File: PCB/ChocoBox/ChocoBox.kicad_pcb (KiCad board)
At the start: 2 copper layers, 101.6 x 61.5 mm, 27 parts, among them J1 DTH22_01, J10 Vout-12V, J11 Conn_01x01, J12 I2C, J13 I2C, J14 Vout-5V-Humidificador, J15 Conn_01x01, J16 Conn_01x01, J17 Conn_01x01, J18 Conn_01x01, J19 DS18B20-A, J2 DTH22_02, J20 DS18B20-B, J21 DS18B20-C, J22 DS18B20-D, J3 DS3231, J4 LCD2004A, J5 microSD, J6 Humidificador, J7 WaterLevel, J8 Vin-12V, J9 Calentador, SW1 BTN1, U1 ESP32-DEVKIT-V1, U2 DCDC_StepDown_LM2596

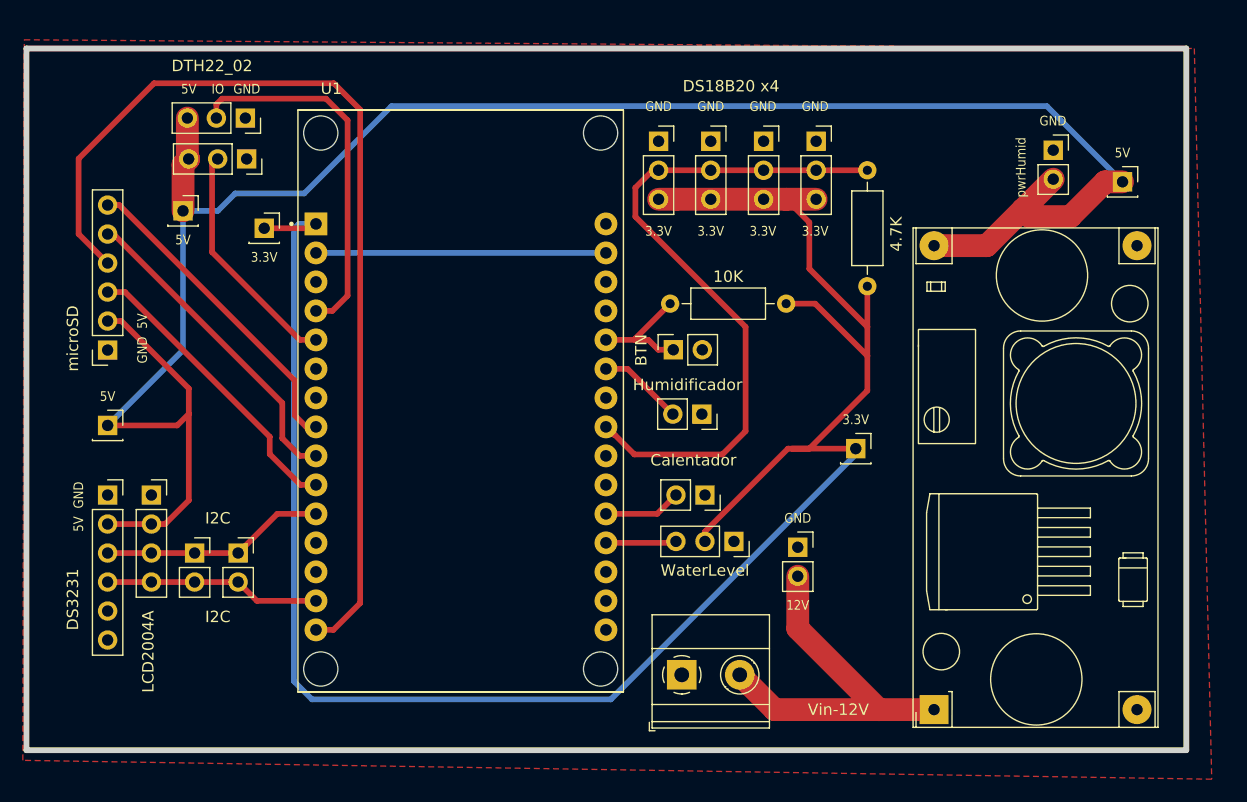
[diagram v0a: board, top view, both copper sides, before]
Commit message: controladores funcionando
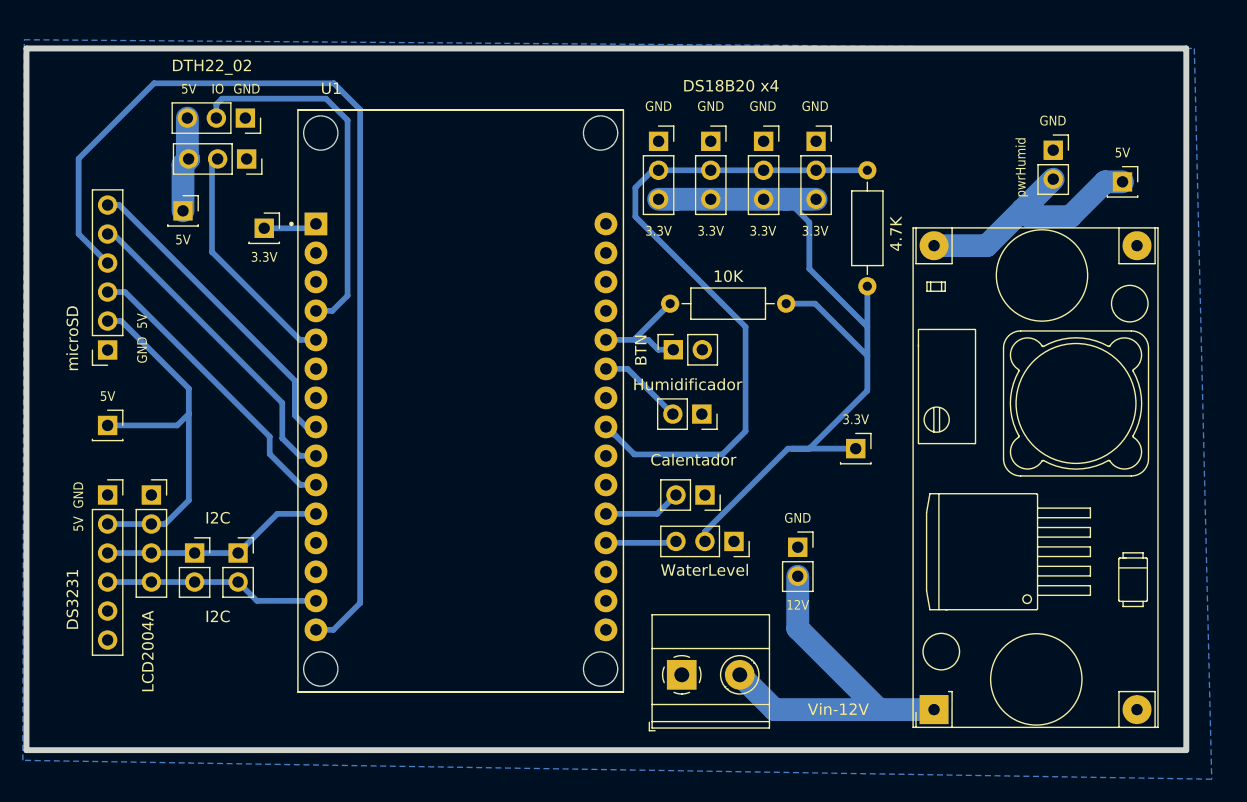
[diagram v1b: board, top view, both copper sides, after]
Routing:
- net +5V: track 176.7 -> 66.3 mm
- net +3.3V: track 176.5 -> 76.0 mm
- net GND: track 25.4 -> 0.00 mm
- added copper zone on B.Cu, net GND
- removed copper zone on F.Cu, net GND

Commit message: Bug fix - App environment.txt
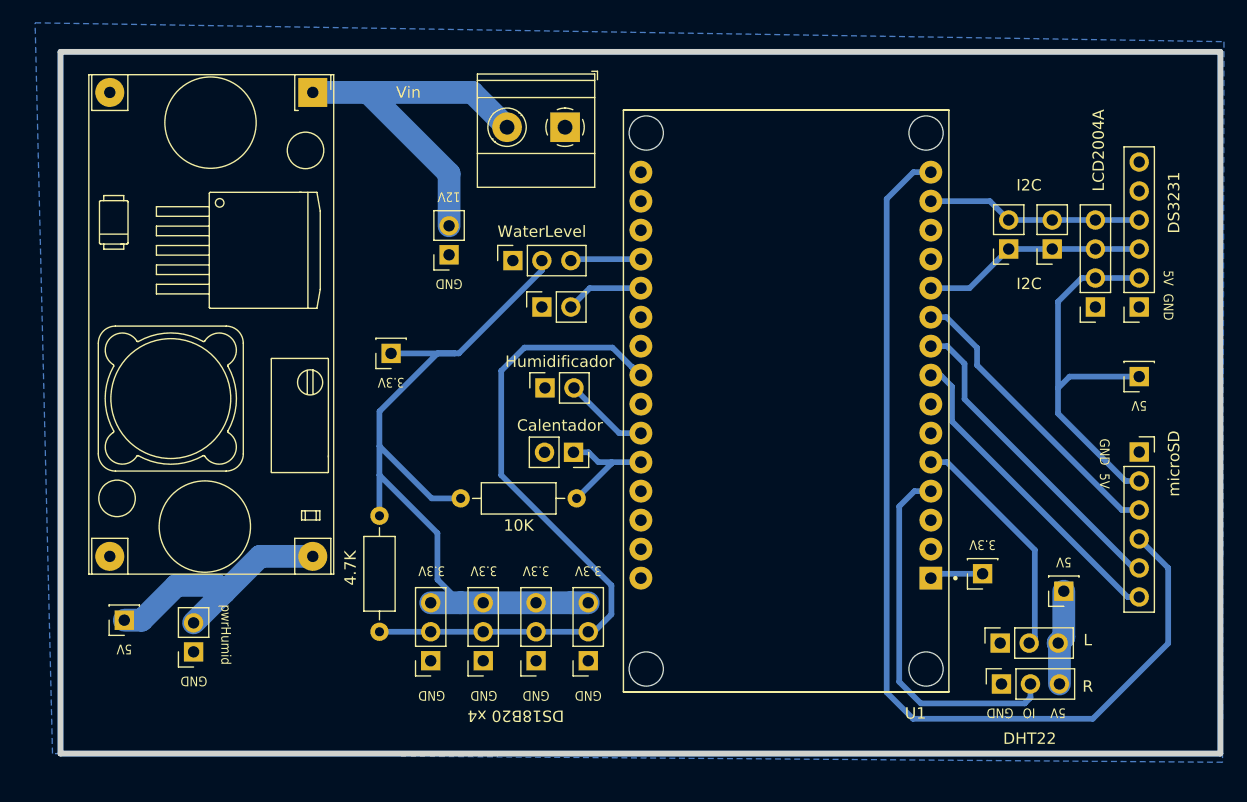
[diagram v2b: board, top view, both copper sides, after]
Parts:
- J2: value DTH22_02 -> R
- J8: value Vin-12V -> Vin
- moved J16 95.5 mm to (70.0, 87.2), turned to 180 degrees
- moved J3 91.8 mm to (158.9, 59.7), turned to 180 degrees
- moved J5 90.8 mm to (158.9, 72.4), turned to 0 degrees
- moved J15 90.5 mm to (158.9, 65.8), turned to 180 degrees
- moved J14 87.2 mm to (76.1, 89.9), turned to 180 degrees
- moved J4 84.3 mm to (155.1, 59.7), turned to 180 degrees
- moved J11 84.0 mm to (152.3, 84.6), turned to 180 degrees
- moved J2 82.7 mm to (146.9, 92.8), turned to 90 degrees
- moved J12 79.7 mm to (151.3, 54.6), turned to 180 degrees
- moved J1 78.5 mm to (146.8, 89.2), turned to 90 degrees
- moved U2 76.7 mm to (86.5, 40.9), turned to -90 degrees
- moved J13 72.6 mm to (147.5, 54.6), turned to 180 degrees
- moved J18 69.8 mm to (145.2, 83.1), turned to 180 degrees
- moved R3 58.8 mm to (92.4, 88.2), turned to 90 degrees
- moved J22 56.7 mm to (96.9, 90.7), turned to 180 degrees
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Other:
- board text added: "Calentador"
- board text added: "DHT22"
- board text added: "L"
- board text removed: "BTN"
